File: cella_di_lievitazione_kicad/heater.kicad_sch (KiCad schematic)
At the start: 8 parts

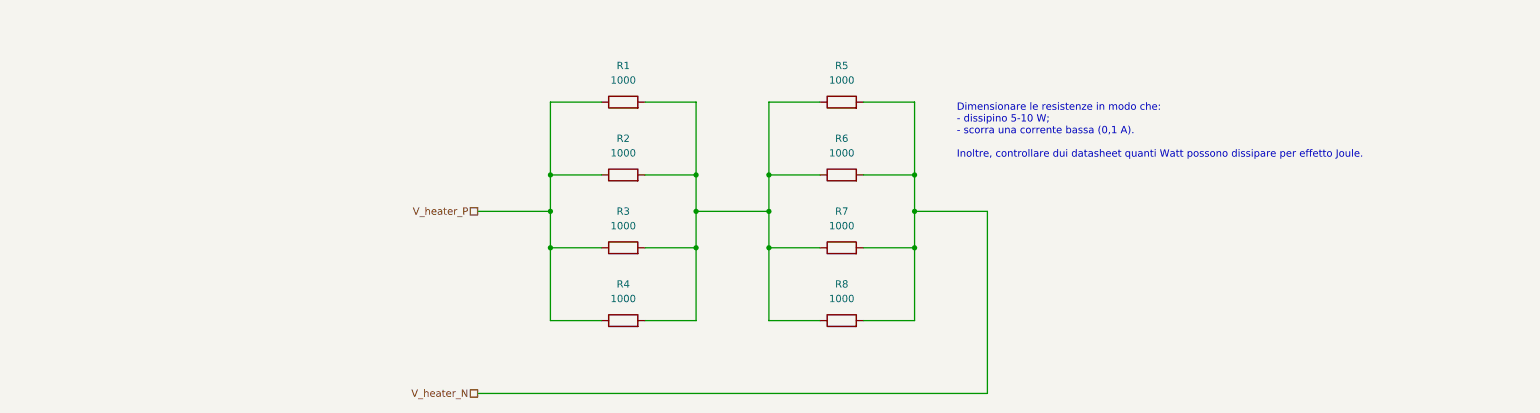
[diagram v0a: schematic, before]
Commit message: no message
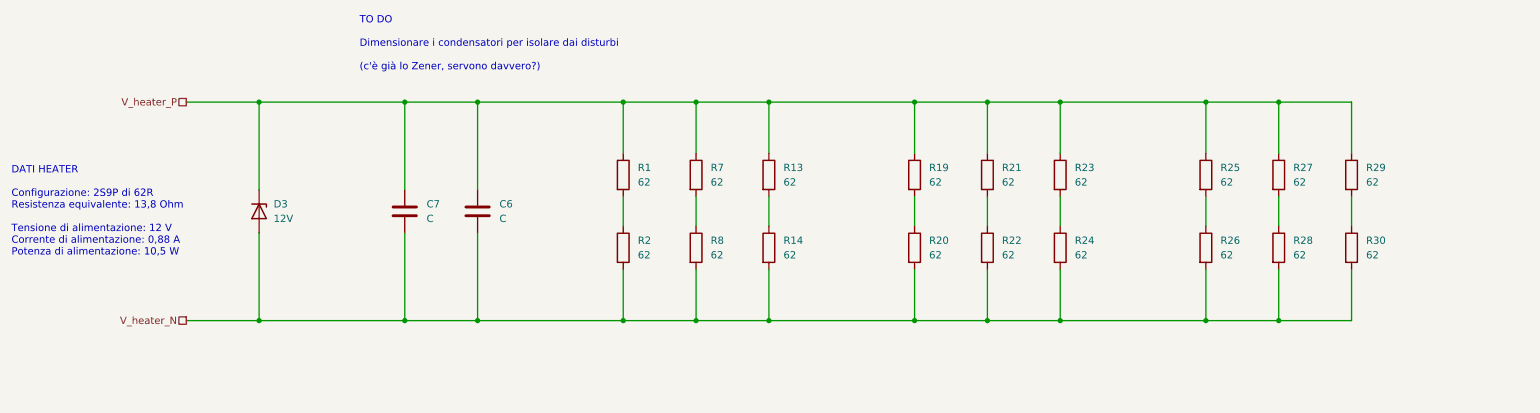
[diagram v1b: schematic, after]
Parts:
- removed R3, R4, R5, R6: 1000, symbol Device:R
- added C6, C7: C, symbol Device:C
- added D3: 12V, symbol Device:D_Zener
- added R13, R14, R19, R20, R21, R22, R23, R24, R25, R26, R27, R28, R29, R30: 62, symbol Device:R
- R1, R2, R7, R8: value 1000 -> 62
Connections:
- net V_heater_N: now also R2.2, C6.2, C7.2, D3.2 (A), R14.2, R20.2, R22.2, R24.2, R26.2, R28.2, R30.2; no longer R7.2
- net V_heater_P: now also R7.1, C6.1, C7.1, D3.1 (K), R13.1, R19.1, R21.1, R23.1, R25.1, R27.1, R29.1; no longer R2.1
- new net: R19.2, R20.1
- new net: R13.2, R14.1
- new net: R21.2, R22.1
- new net: R27.2, R28.1
- new net: R29.2, R30.1
- new net: R7.2, R8.1
- new net: R23.2, R24.1
- new net: R1.2, R2.1
- new net: R25.2, R26.1
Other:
- note added: "DATI HEATER Configurazione: 2S9P di 62R Resistenza equivalente: 13,8 Ohm Tensione di alimentazione: 12 V Corrente di alimentazione: 0,88 A Potenza di alimentazione: 10,5 W"
- note added: "TO DO Dimensionare i condensatori per isolare dai disturbi (c'è già lo Zener, servono davvero?)"
- note removed: "Dimensionare le resistenze in modo che: - dissipino 5-10 W; - scorra una corrente bassa (0,1 A). Inoltre, controllare dui datasheet quanti Watt possono dissipare per effetto Joule."
